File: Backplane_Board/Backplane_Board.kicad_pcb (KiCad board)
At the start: 4 copper layers, 179.7 x 127.9 mm, 175 parts, among them J1 XT60, J10 Conn_01x02_Pin, J11 Conn_01x02_Pin, J12 Conn_01x02_Pin, J13 Conn_01x02_Pin, J14 Conn_01x02_Pin, J15 Conn_01x02_Pin, J16 Conn_01x02_Pin, J17 Conn_01x02_Pin, J18 Conn_01x02_Pin, J19 Conn_01x02_Pin, J2 XT60, J20 Conn_01x02_Pin, J21 Conn_01x02_Pin, J22 Conn_01x02_Pin, J23 Conn_01x02_Pin, J24 Conn_01x02_Pin, J25 Conn_01x02_Pin, J26 Conn_01x02_Pin, J27 Conn_01x03_Pin, J28 Conn_01x03_Pin, J29 Conn_01x03_Pin, J3 Conn_01x02_Pin, J30 BM03B-SRSS-TB, J31 Conn_01x04, J32 Conn_01x05_Socket, J33 BM03B-SRSS-TB, J34 Connector_PinHeader_2.54mm:Pi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, J35 Connector_PinHeader_2.54mm:Pi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, J36 Conn_01x03_Pin, J37 Conn_01x02, J38 Conn_01x02, J39 Conn_01x02, J4 Conn_01x07_Female, J40 Conn_01x02, J41 Conn_01x02, J42 Conn_01x02, J5 Conn_01x02_Pin, J6 Conn_01x02_Pin, J7 Conn_01x02_Pin, J8 Conn_01x02_Pin, J9 Conn_01x02_Pin, Q1 FDMS86163P, Q2 FDMS86163P, Q3 SI7615ADN-T1-GE3, Q4 ZXMN3A14F, Q5 ZXMN3A14F, Q6 ZXMN3A14F, Q7 ZXMN3A14F, Q8 ZXMN3A14F, Q9 ZXMN3A14F, SW1 SW_DPST_x2, U1 ZXTR2005ZQ-13, U2 PINA740AIREMR, U3 PKJ7213WPI, U4 PKJ7213WPI, U5 PKU3511SPI, U6 Pico

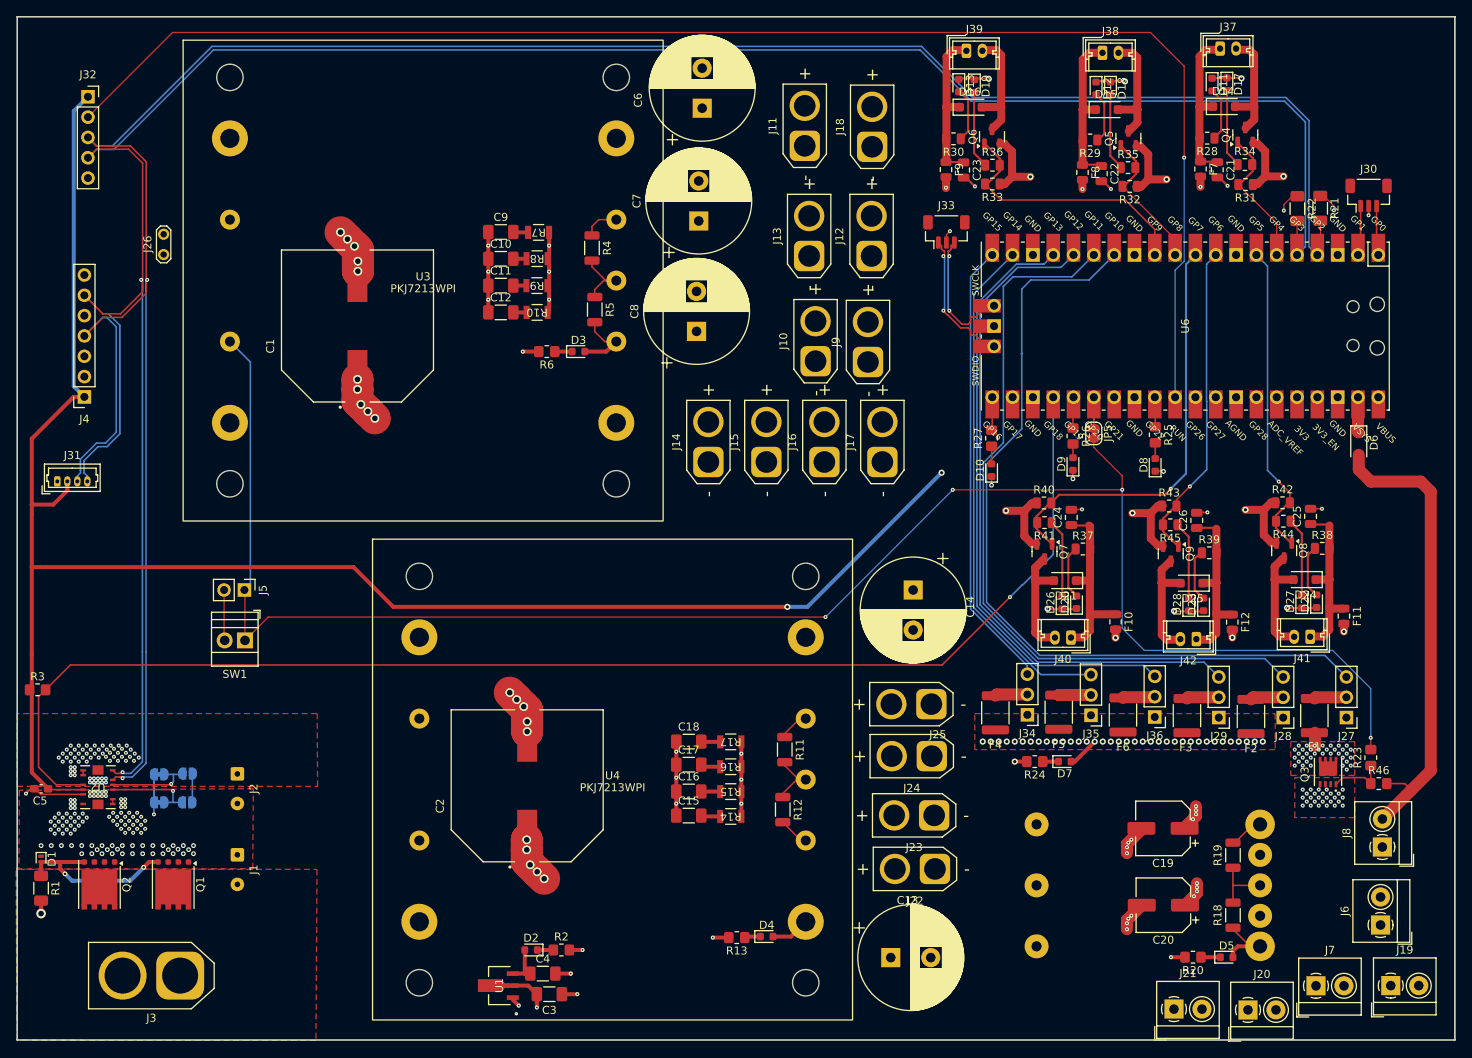
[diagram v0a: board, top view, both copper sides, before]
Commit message: few drc errors left - must fix fet footprints
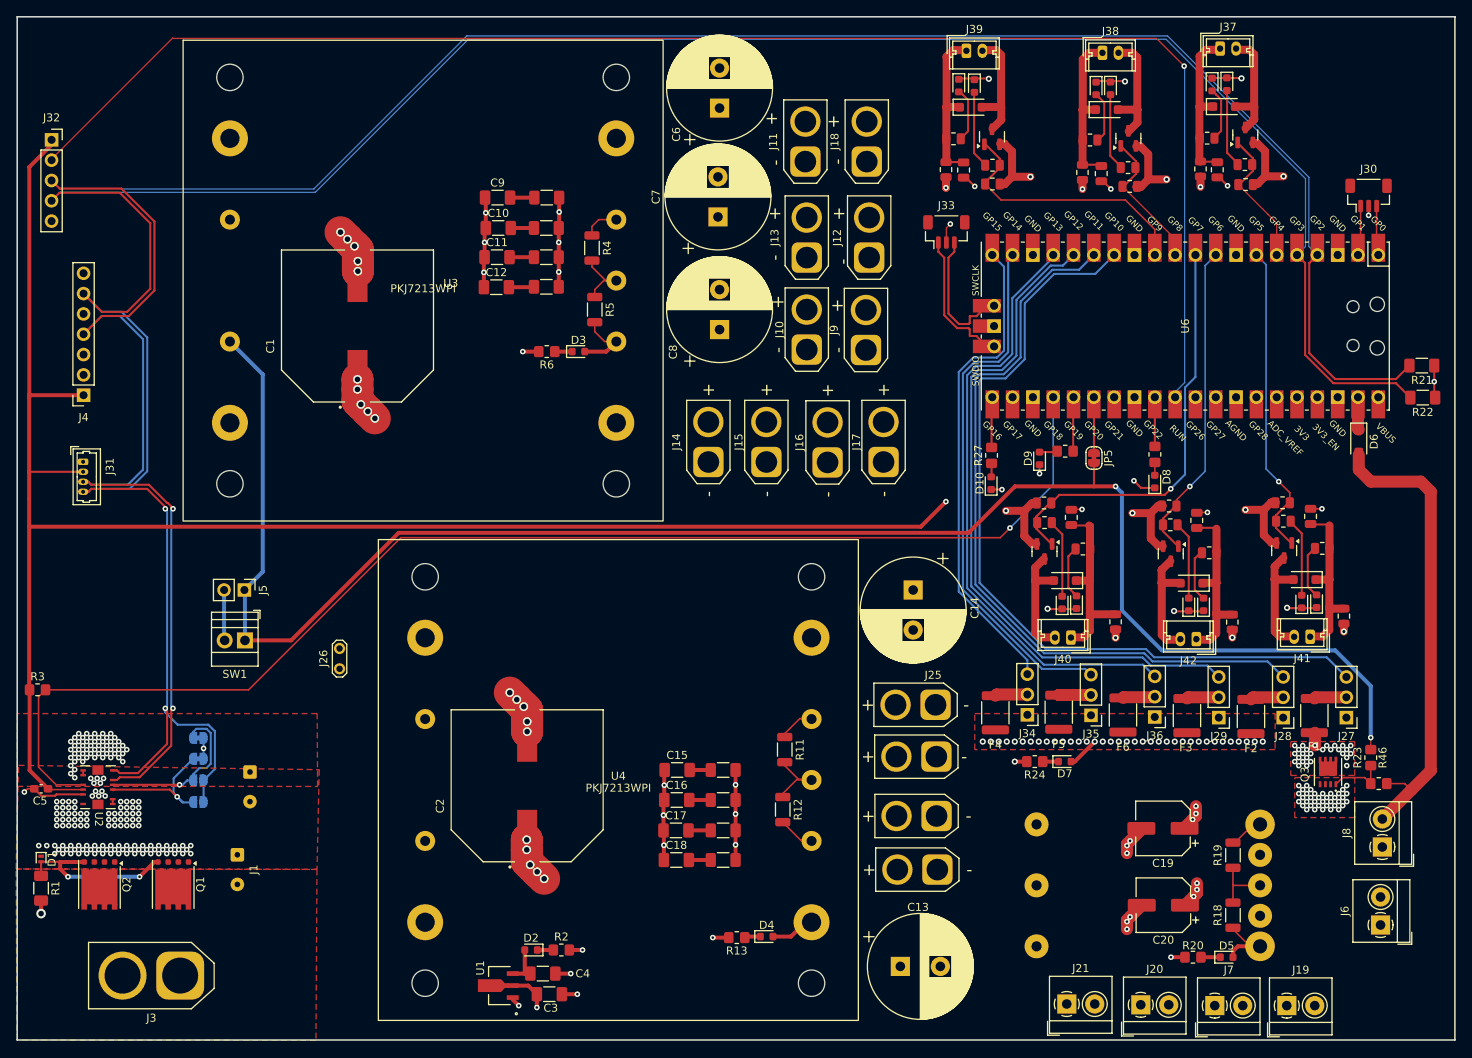
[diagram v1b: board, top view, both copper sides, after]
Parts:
- moved J26 56.3 mm to (71.6, 104.9)
- moved R22 28.4 mm to (207.0, 71.0), turned to 180 degrees
- moved R21 23.4 mm to (206.9, 67.0), turned to 180 degrees
- moved C18 14.9 mm to (113.7, 128.8)
- moved R17 14.7 mm to (119.7, 128.7)
- moved J20 13.4 mm to (171.8, 146.9)
- moved J21 13.4 mm to (162.5, 146.8)
- moved J19 13.2 mm to (190.0, 147.0)
- moved J7 12.9 mm to (181.0, 147.0)
- moved C17 8.37 mm to (113.7, 125.1)
- moved R16 7.90 mm to (119.7, 125.0)
- moved JP3 7.33 mm to (54.0, 116.2), turned to 0 degrees
- moved J32 7.05 mm to (35.6, 38.8)
- moved JP4 6.69 mm to (54.0, 113.5), turned to 0 degrees
- moved R14 5.97 mm to (119.7, 117.5)
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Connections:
- JP1 pad 2: SCL -> I2C-
- JP2 pad 2: SCL -> I2C-
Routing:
- net I2C-: track 309.6 -> 346.4 mm
- net I2C+: track 312.0 -> 333.5 mm
- net +3.3V: track 231.7 -> 221.3 mm, vias 4 -> 2
- net A0: track 11.0 -> 21.0 mm
- net RUN: track 185.0 -> 191.3 mm
- net A1: track 11.9 -> 17.7 mm
- net ALERT: track 169.1 -> 164.0 mm
- net KillSW: track 224.2 -> 219.6 mm, vias 4 -> 2
- net SERVO5: track 56.5 -> 60.6 mm
- net SCL: track 3.76 -> 0.00 mm
- net esc_status: track 3.88 -> 6.96 mm
- net Net-(U6-GPIO19): track 3.88 -> 6.87 mm
- net Net-(U6-GPIO22): track 3.85 -> 6.24 mm
- net SERVO4: track 64.2 -> 66.6 mm
- net Net-(U6-GPIO16): track 4.16 -> 6.31 mm
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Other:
- rule pad_to_mask_clearance: 0 -> 0.0508
